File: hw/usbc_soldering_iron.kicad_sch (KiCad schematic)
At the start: 78 parts, among them J1 USB_C_Receptacle_USB2.0_14P, J10 TIP_L, J11 TIP_H, J12 TIP_K, J13 TIP_L, J14 TIP_H, J15 TIP_K, J16 TIP_L, J2 DBG, J3 LED RING, J4 OLED, J5 TIP_H, J6 TIP_K, J7 TIP_L, J8 TIP_H, J9 TIP_K, SW1 B2, SW2 B1, SW3 BS, U1 CH32V203GxUx, U2 FUSB302BMPX, U3 TPD4E05U06DQA, U4 AP63201WU, U5 SC7A20, U6 TPA191Ax, U7 TLV333IDBVR, U9 TMP102xxDRL

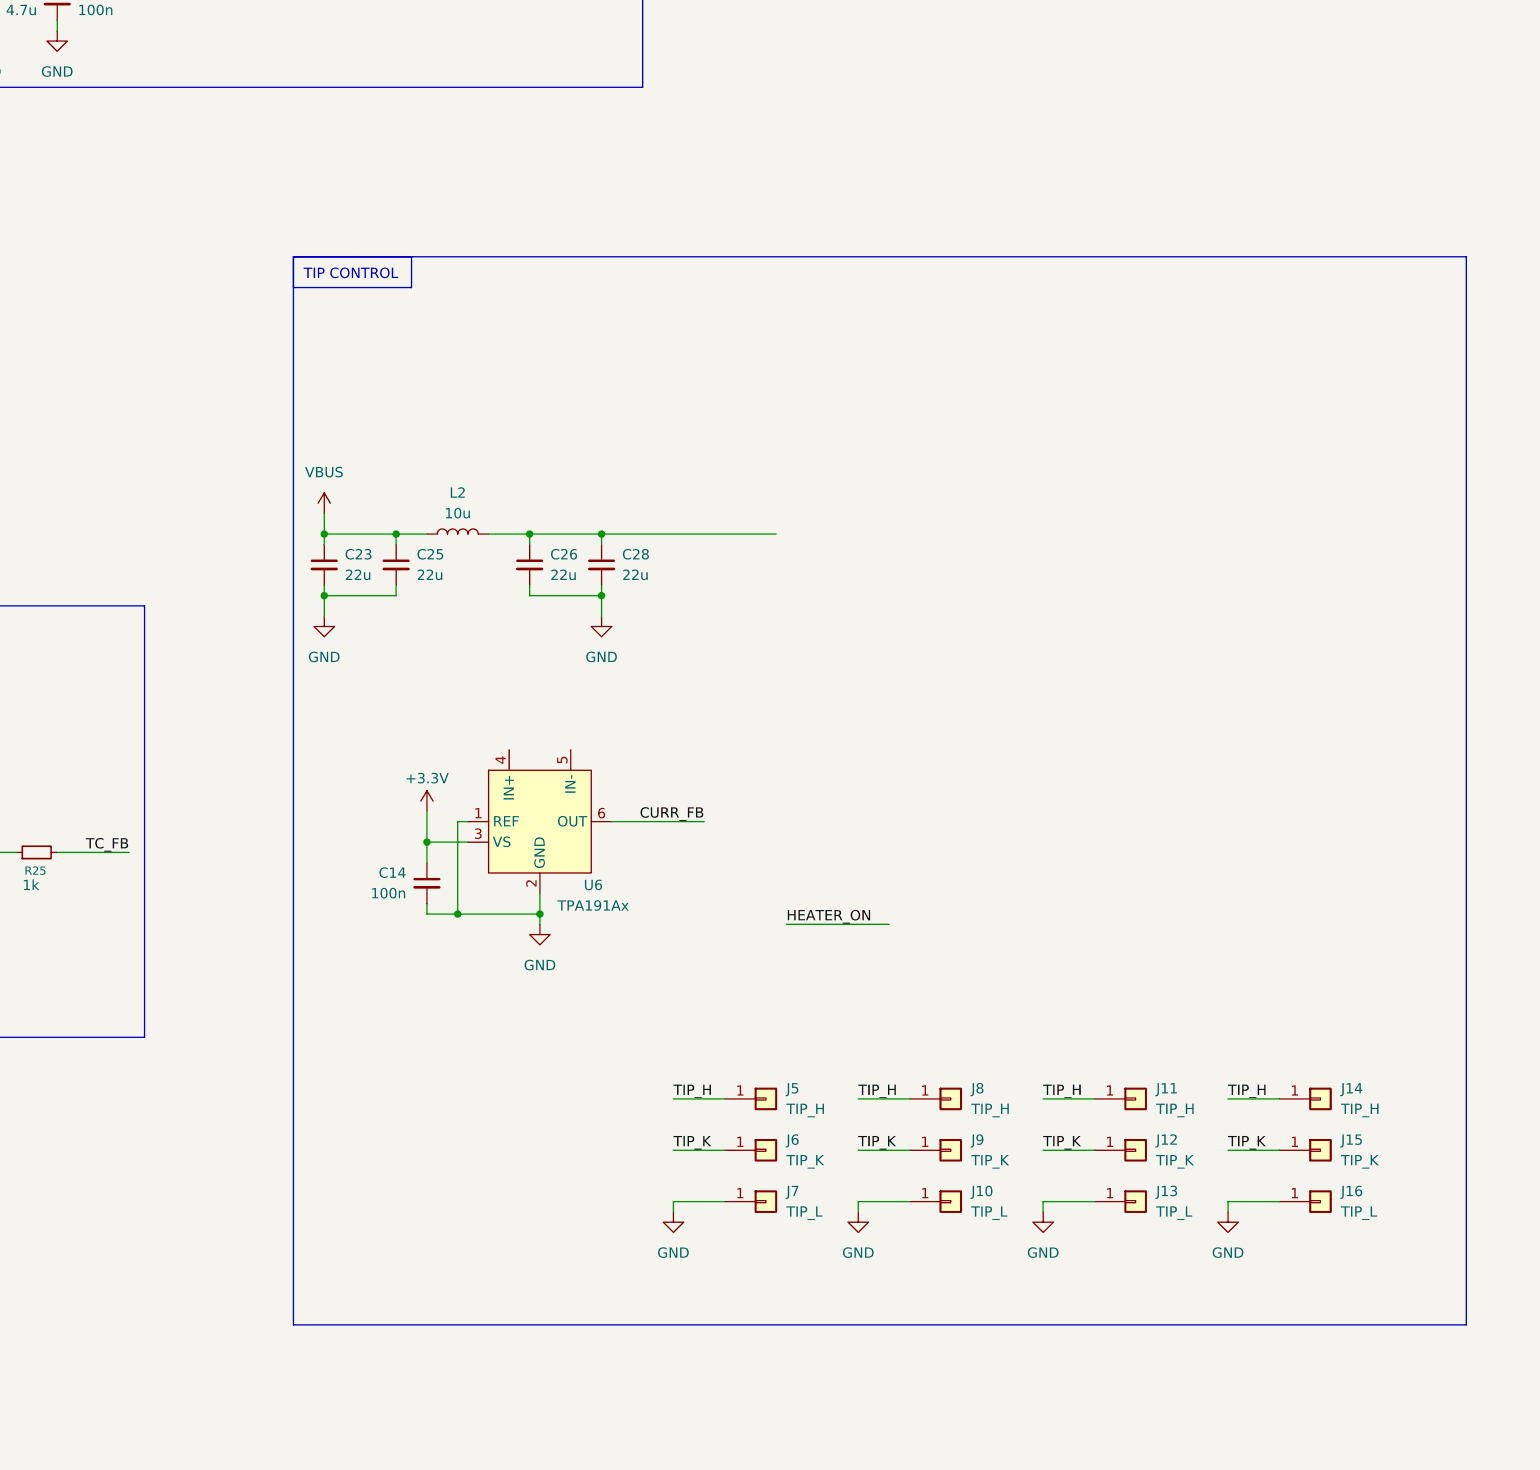
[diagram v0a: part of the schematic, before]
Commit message: mosfets and driver
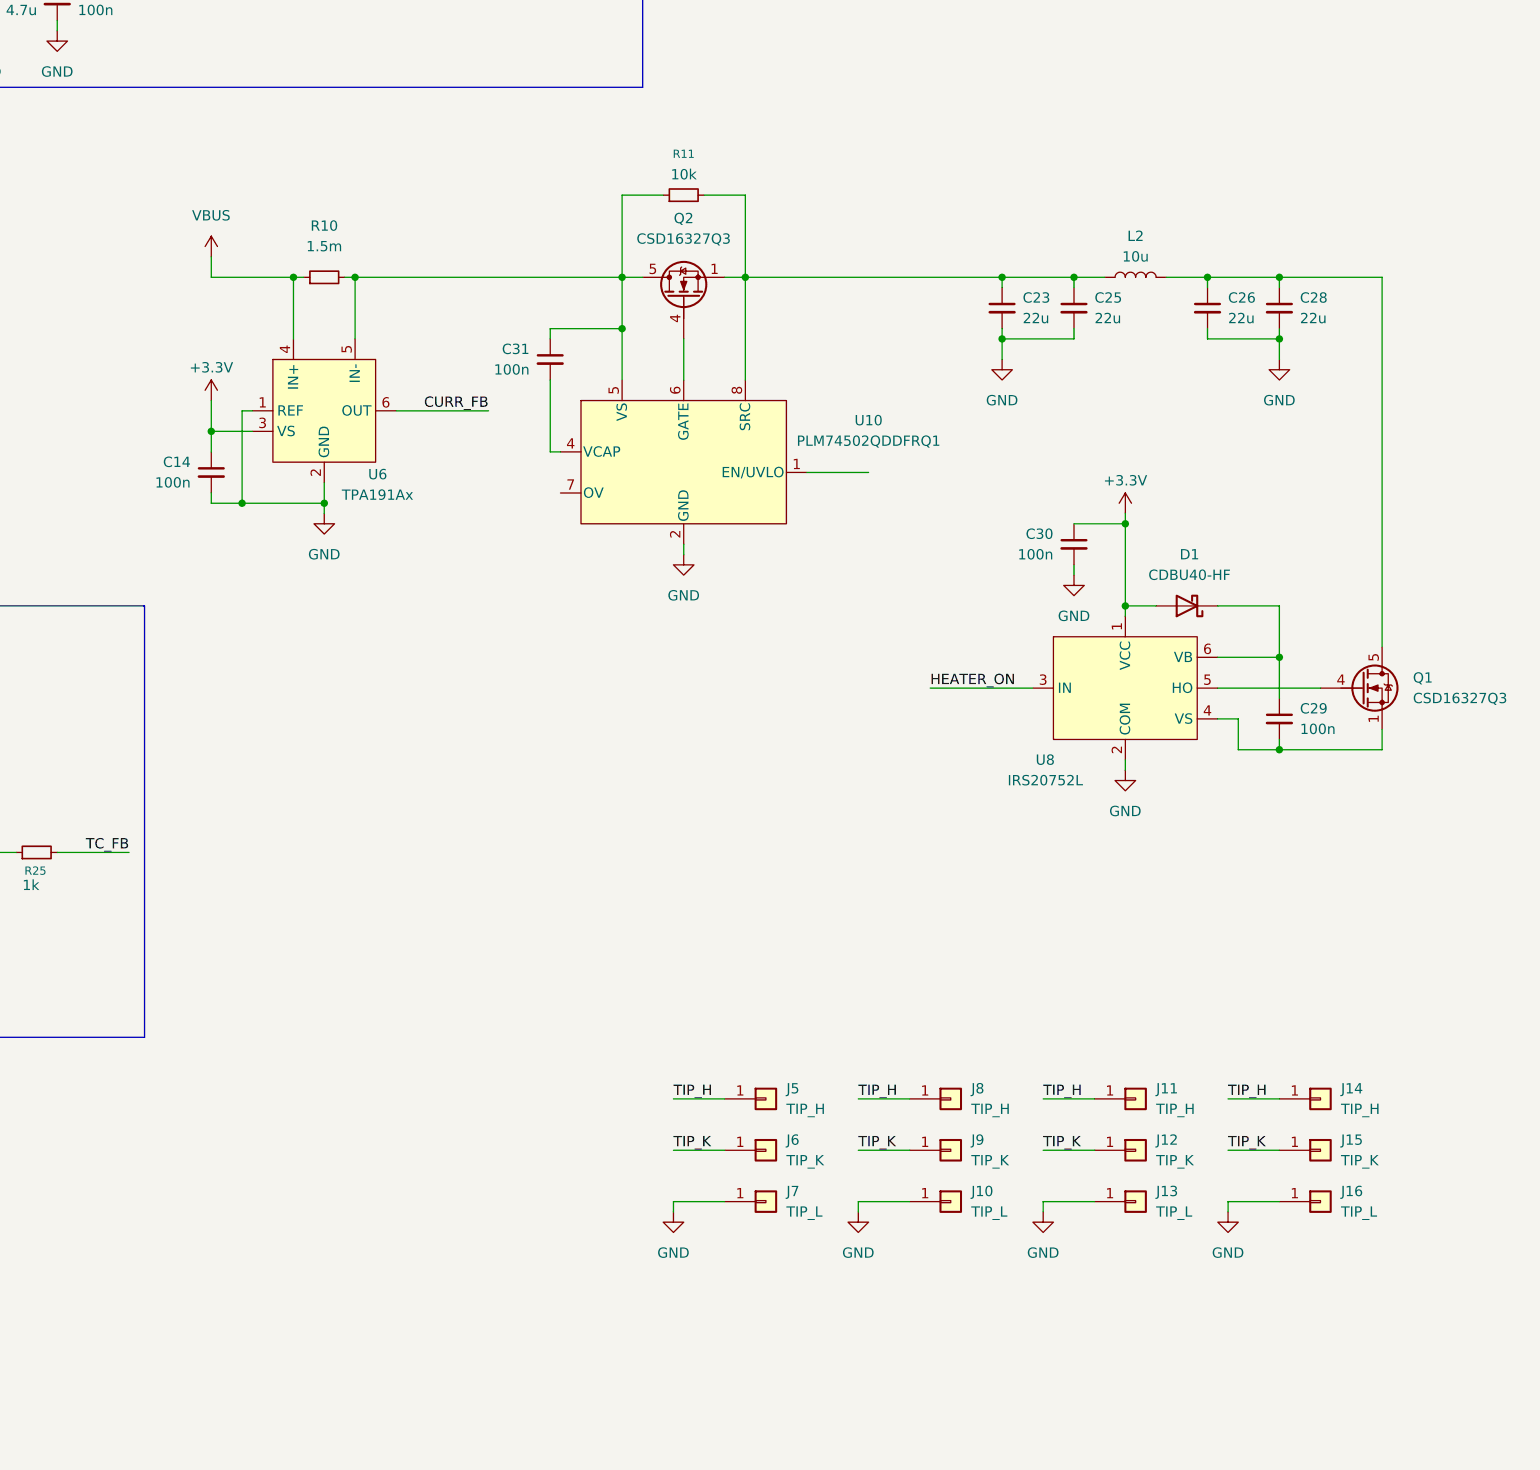
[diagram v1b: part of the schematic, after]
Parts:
- added C29, C30, C31: 100n, Capacitor_SMD:C_0603_1608Metric, symbol Device:C_Small
- added D1: CDBU40-HF, Diode_SMD:D_0603_1608Metric, symbol Diode:CDBU40-HF
- added Q1, Q2: CSD16327Q3, Package_SON:VSON-8_3.3x3.3mm_P0.65mm_NexFET, symbol Transistor_FET:CSD16327Q3
- added R10: 1.5m, Resistor_SMD:R_1206_3216Metric, symbol Device:R_Small
- added R11: 10k, Capacitor_SMD:C_0603_1608Metric, symbol Device:R_Small
- added U10: PLM74502QDDFRQ1, Package_TO_SOT_SMD:SOT-23-8, symbol custom_library:PLM74502QDDFRQ1
- added U8: IRS20752L, Package_TO_SOT_SMD:SOT-23-6, symbol custom_library:IRS20752L
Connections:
- net +3.3V: now also C30.1, D1.2 (A), U8.1 (VCC)
- net GND: now also C30.2, U10.2 (GND), U8.2 (COM)
- net HEATER_ON: now also U8.3 (IN)
- net VBUS: now also U6.4 (IN+), R10.1; no longer C23.1, C25.1, L2.1
- net at U6.5 (IN-): now also C31.1, Q2.5 (D), R10.2, R11.1, U10.5 (VS)
- net at C26.1, C28.1, L2.2: now also Q1.5 (D)
- new net: C31.2, U10.4 (VCAP)
- new net: Q2.4 (G), U10.6 (GATE)
- new net: C23.1, C25.1, L2.1, Q2.1 (S), Q2.2 (S), Q2.3 (S), R11.2, U10.8 (SRC)
- new net: C29.1, D1.1 (K), U8.6 (VB)
- new net: C29.2, Q1.1 (S), Q1.2 (S), Q1.3 (S), U8.4 (VS)
- new net: Q1.4 (G), U8.5 (HO)
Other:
- note removed: "TIP CONTROL"
- moved on the sheet: C14, C23, C25, C26, C28, L2, U6

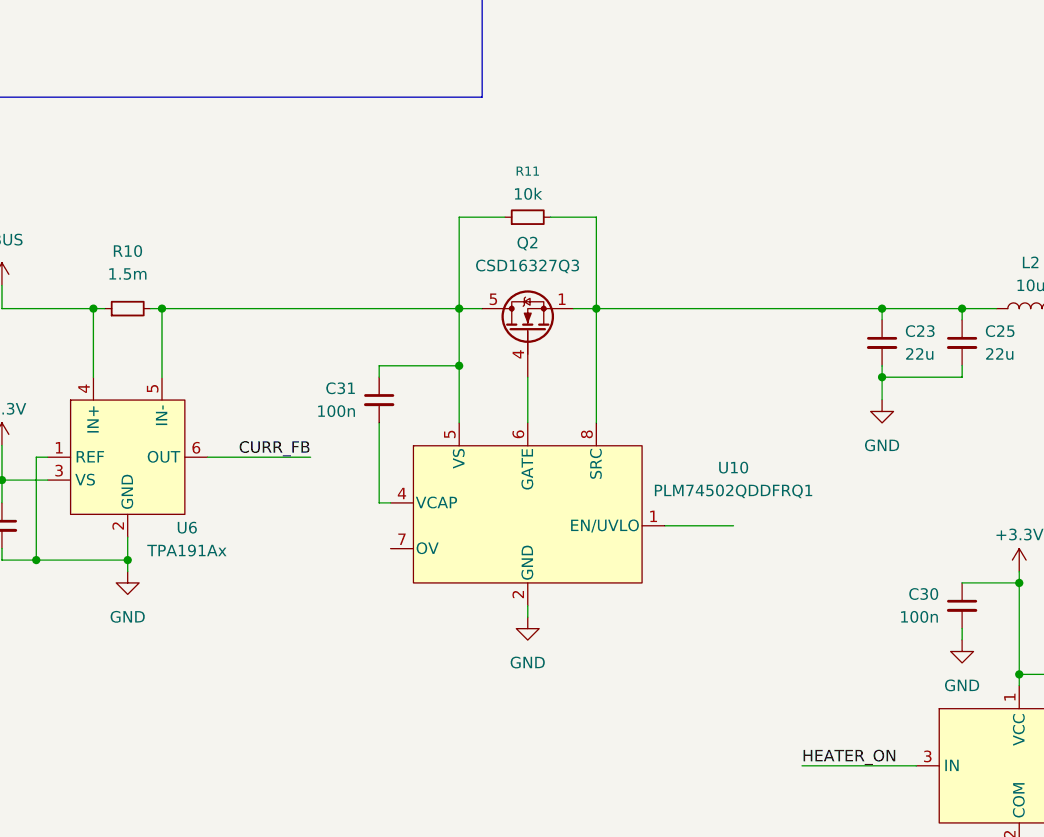
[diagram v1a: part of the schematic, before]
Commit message: different mosfets
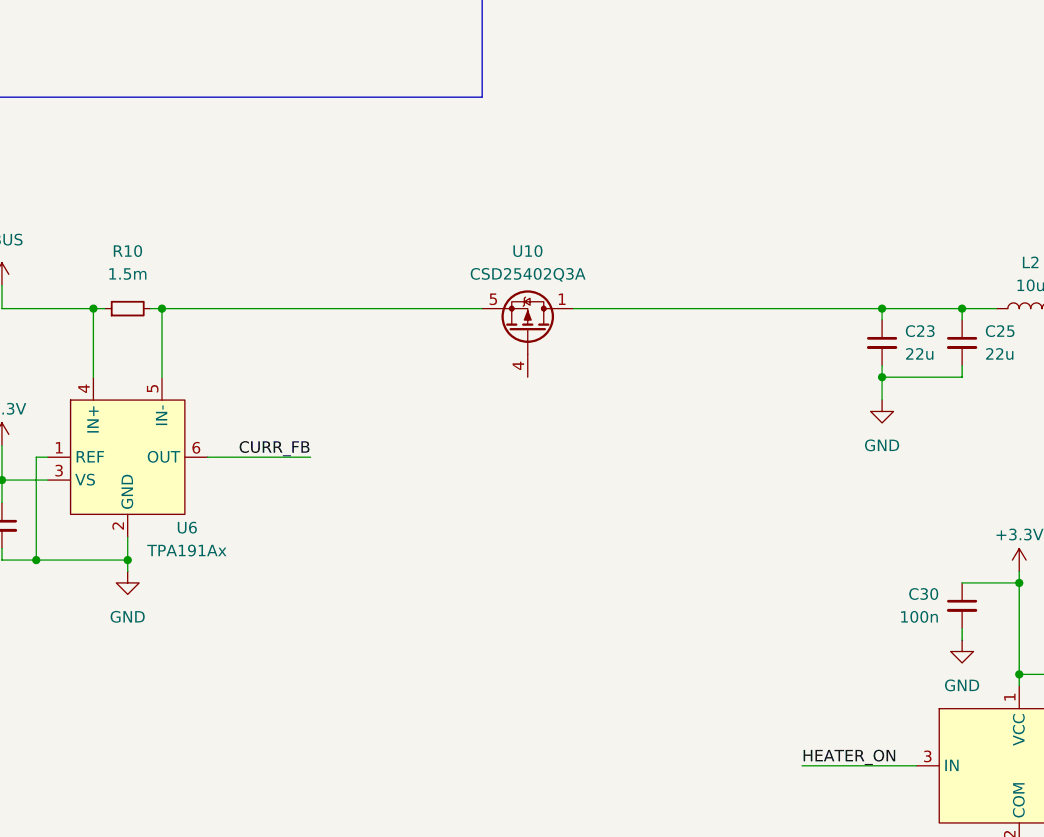
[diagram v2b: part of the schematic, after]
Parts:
- removed C31: 100n, Capacitor_SMD:C_0603_1608Metric, symbol Device:C_Small
- removed Q2: CSD16327Q3, Package_SON:VSON-8_3.3x3.3mm_P0.65mm_NexFET, symbol Transistor_FET:CSD16327Q3
- removed R11: 10k, Capacitor_SMD:C_0603_1608Metric, symbol Device:R_Small
- removed U10: PLM74502QDDFRQ1, Package_TO_SOT_SMD:SOT-23-8, symbol custom_library:PLM74502QDDFRQ1
- added U10: CSD25402Q3A, Package_SON:VSON-8_3.3x3.3mm_P0.65mm_NexFET, symbol Transistor_FET:CSD25402Q3A
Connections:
- net at R10.2, U6.5 (IN-): now also U10.5 (S)
- net at C23.1, C25.1, L2.1: now also U10.1 (D), U10.2 (D), U10.3 (D)
